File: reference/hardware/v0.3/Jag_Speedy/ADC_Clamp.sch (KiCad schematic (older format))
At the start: 1 part, among them IC10 SP720APP

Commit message: Rationalise level shifting
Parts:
- added IC12: SP720APP, Package_DIP:DIP-16_W7.62mm, symbol Jag_Speedy-rescue:SP720APP-SP720APP-Jag_Speedy-rescue
- added R1, R2, R7, R8: 180k, Resistor_THT:R_Axial_DIN0207_L6.3mm_D2.5mm_P2.54mm_Vertical, symbol Device:R
- added R3, R4, R5, R6: 330k, Resistor_THT:R_Axial_DIN0207_L6.3mm_D2.5mm_P2.54mm_Vertical, symbol Device:R
- added U1: LMV324, Package_DIP:DIP-14_W7.62mm_Socket, symbol Amplifier_Operational:LMV324
- IC10: symbol Jag_Speedy-rescue:SP720APP-SP720APP -> Jag_Speedy-rescue:SP720APP-SP720APP-Jag_Speedy-rescue
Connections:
- net ADCClamp05: now also IC12.1 (IN_1); no longer IC10.5 (IN_5)
- net ADCClamp09: now also IC12.9 (IN_8); no longer IC10.10 (IN_9)
- net ADCClamp10: now also IC12.10 (IN_9); no longer IC10.11 (IN_10)
- net ADCClamp11: now also IC12.11 (IN_10); no longer IC10.12 (IN_11)
- net SignalGnd: now also IC12.8 (V-), R3.2, R4.2, R5.1, R6.1, U1.11 (V-)
- new net: R1.2, R4.1, U1.12 (+)
- new net: R6.2, R8.1, U1.10 (+)
- new net: R2.2, R3.1, U1.5 (+)
- new net: R5.2, R7.1, U1.3 (+)
- new net 3V3: IC12.16 (V+), U1.4 (V+)
- new net Barro-Signal-3.3V: U1.6 (-), U1.7
- new net Barro-Signal-5V: R2.1
- new net MAP-Signal-3.3V: U1.13 (-), U1.14
- new net MAP-Signal-5V: R1.1
- new net O2-Signal-3.3V: U1.1, U1.2 (-)
- new net O2-Signal-5V: R7.2
- new net TPS-Signal-3.3V: U1.8, U1.9 (-)
- new net TPS-Signal-5V: R8.2
- no-connect marks 3 -> 17
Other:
- moved on the sheet: IC10

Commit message: SMD Update
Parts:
- IC10, IC12: footprint Package_DIP:DIP-16_W7.62mm -> Package_SO:SOIC-16_3.9x9.9mm_P1.27mm
- R1, R2, R3, R4, R5, R6, R7, R8: footprint Resistor_THT:R_Axial_DIN0207_L6.3mm_D2.5mm_P2.54mm_Vertical -> Resistor_SMD:R_0805_2012Metric
- U1: footprint Package_DIP:DIP-14_W7.62mm_Socket -> Package_SO:SO-14_5.3x10.2mm_P1.27mm
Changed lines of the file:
@@
 F 0 "IC10" H 2600 1815 50  0000 C CNN
 F 1 "SP720APP" H 2600 1724 50  0000 C CNN
-F 2 "Package_DIP:DIP-16_W7.62mm" H 3050 1650 50  0001 L CNN
+F 2 "Package_SO:SOIC-16_3.9x9.9mm_P1.27mm" H 3050 1650 50  0001 L CNN
 F 3 "https://componentsearchengine.com/Datasheets/1/SP720APP.pdf" H 3050 1550 50  0001 L CNN
 F 4 "TVS Diode Arrays 14 CH DIODE ARRAY" H 3050 1450 50  0001 L CNN "Description"
@@
 F 0 "IC12" H 2600 3115 50  0000 C CNN
 F 1 "SP720APP" H 2600 3024 50  0000 C CNN
-F 2 "Package_DIP:DIP-16_W7.62mm" H 3050 2950 50  0001 L CNN
+F 2 "Package_SO:SOIC-16_3.9x9.9mm_P1.27mm" H 3050 2950 50  0001 L CNN
 F 3 "https://componentsearchengine.com/Datasheets/1/SP720APP.pdf" H 3050 2850 50  0001 L CNN
 F 4 "TVS Diode Arrays 14 CH DIODE ARRAY" H 3050 2750 50  0001 L CNN "Description"
@@
 F 0 "U1" V 6945 3600 50  0000 C CNN
 F 1 "LMV324" V 6854 3600 50  0000 C CNN
-F 2 "Package_DIP:DIP-14_W7.62mm_Socket" H 6800 3700 50  0001 C CNN
+F 2 "Package_SO:SO-14_5.3x10.2mm_P1.27mm" H 6800 3700 50  0001 C CNN
 F 3 "http://www.ti.com/lit/ds/symlink/lmv324.pdf" H 6900 3800 50  0001 C CNN
 	5    6850 3600
@@
 F 0 "U1" V 6354 3180 50  0000 L CNN
 F 1 "LMV324" V 6445 3180 50  0000 L CNN
-F 2 "Package_DIP:DIP-14_W7.62mm_Socket" H 6350 3050 50  0001 C CNN
+F 2 "Package_SO:SO-14_5.3x10.2mm_P1.27mm" H 6350 3050 50  0001 C CNN
 F 3 "http://www.ti.com/lit/ds/symlink/lmv324.pdf" H 6450 3150 50  0001 C CNN
 	4    6400 2950
@@
 F 0 "U1" V 7154 3180 50  0000 L CNN
 F 1 "LMV324" V 7245 3180 50  0000 L CNN
-F 2 "Package_DIP:DIP-14_W7.62mm_Socket" H 7150 3050 50  0001 C CNN
+F 2 "Package_SO:SO-14_5.3x10.2mm_P1.27mm" H 7150 3050 50  0001 C CNN
 F 3 "http://www.ti.com/lit/ds/symlink/lmv324.pdf" H 7250 3150 50  0001 C CNN
 	3    7200 2950
@@
 F 0 "U1" V 6354 2080 50  0000 L CNN
 F 1 "LMV324" V 6445 2080 50  0000 L CNN
-F 2 "Package_DIP:DIP-14_W7.62mm_Socket" H 6350 1950 50  0001 C CNN
+F 2 "Package_SO:SO-14_5.3x10.2mm_P1.27mm" H 6350 1950 50  0001 C CNN
 F 3 "http://www.ti.com/lit/ds/symlink/lmv324.pdf" H 6450 2050 50  0001 C CNN
 	2    6400 1850
@@
 F 0 "U1" V 7154 2080 50  0000 L CNN
 F 1 "LMV324" V 7245 2080 50  0000 L CNN
-F 2 "Package_DIP:DIP-14_W7.62mm_Socket" H 7150 1950 50  0001 C CNN
+F 2 "Package_SO:SO-14_5.3x10.2mm_P1.27mm" H 7150 1950 50  0001 C CNN
 F 3 "http://www.ti.com/lit/ds/symlink/lmv324.pdf" H 7250 2050 50  0001 C CNN
 	1    7200 1850
@@
 F 0 "R8" V 7707 2550 50  0000 C CNN
 F 1 "180k" V 7616 2550 50  0000 C CNN
-F 2 "Resistor_THT:R_Axial_DIN0207_L6.3mm_D2.5mm_P2.54mm_Vertical" V 7430 2550 50  0001 C CNN
+F 2 "Resistor_SMD:R_0805_2012Metric" V 7430 2550 50  0001 C CNN
 F 3 "~" H 7500 2550 50  0001 C CNN
 	1    7500 2550
@@
 F 0 "R6" V 7307 2550 50  0000 C CNN
 F 1 "330k" V 7216 2550 50  0000 C CNN
-F 2 "Resistor_THT:R_Axial_DIN0207_L6.3mm_D2.5mm_P2.54mm_Vertical" V 7030 2550 50  0001 C CNN
+F 2 "Resistor_SMD:R_0805_2012Metric" V 7030 2550 50  0001 C CNN
 F 3 "~" H 7100 2550 50  0001 C CNN
 	1    7100 2550
@@
 F 0 "R4" V 6907 2550 50  0000 C CNN
 F 1 "330k" V 6816 2550 50  0000 C CNN
-F 2 "Resistor_THT:R_Axial_DIN0207_L6.3mm_D2.5mm_P2.54mm_Vertical" V 6630 2550 50  0001 C CNN
+F 2 "Resistor_SMD:R_0805_2012Metric" V 6630 2550 50  0001 C CNN
 F 3 "~" H 6700 2550 50  0001 C CNN
 	1    6700 2550
@@
 F 0 "R1" V 6407 2550 50  0000 C CNN
 F 1 "180k" V 6316 2550 50  0000 C CNN
-F 2 "Resistor_THT:R_Axial_DIN0207_L6.3mm_D2.5mm_P2.54mm_Vertical" V 6130 2550 50  0001 C CNN
+F 2 "Resistor_SMD:R_0805_2012Metric" V 6130 2550 50  0001 C CNN
 F 3 "~" H 6200 2550 50  0001 C CNN
 	1    6200 2550
@@
 F 0 "R3" V 6907 1450 50  0000 C CNN
 F 1 "330k" V 6816 1450 50  0000 C CNN
-F 2 "Resistor_THT:R_Axial_DIN0207_L6.3mm_D2.5mm_P2.54mm_Vertical" V 6630 1450 50  0001 C CNN
+F 2 "Resistor_SMD:R_0805_2012Metric" V 6630 1450 50  0001 C CNN
 F 3 "~" H 6700 1450 50  0001 C CNN
 	1    6700 1450
@@
 F 0 "R2" V 6457 1450 50  0000 C CNN
 F 1 "180k" V 6366 1450 50  0000 C CNN
-F 2 "Resistor_THT:R_Axial_DIN0207_L6.3mm_D2.5mm_P2.54mm_Vertical" V 6180 1450 50  0001 C CNN
+F 2 "Resistor_SMD:R_0805_2012Metric" V 6180 1450 50  0001 C CNN
 F 3 "~" H 6250 1450 50  0001 C CNN
 	1    6250 1450
@@
 F 0 "R7" V 7707 1450 50  0000 C CNN
 F 1 "180k" V 7616 1450 50  0000 C CNN
-F 2 "Resistor_THT:R_Axial_DIN0207_L6.3mm_D2.5mm_P2.54mm_Vertical" V 7430 1450 50  0001 C CNN
+F 2 "Resistor_SMD:R_0805_2012Metric" V 7430 1450 50  0001 C CNN
 F 3 "~" H 7500 1450 50  0001 C CNN
 	1    7500 1450
@@
 F 0 "R5" V 7307 1450 50  0000 C CNN
 F 1 "330k" V 7216 1450 50  0000 C CNN
-F 2 "Resistor_THT:R_Axial_DIN0207_L6.3mm_D2.5mm_P2.54mm_Vertical" V 7030 1450 50  0001 C CNN
+F 2 "Resistor_SMD:R_0805_2012Metric" V 7030 1450 50  0001 C CNN
 F 3 "~" H 7100 1450 50  0001 C CNN
 	1    7100 1450

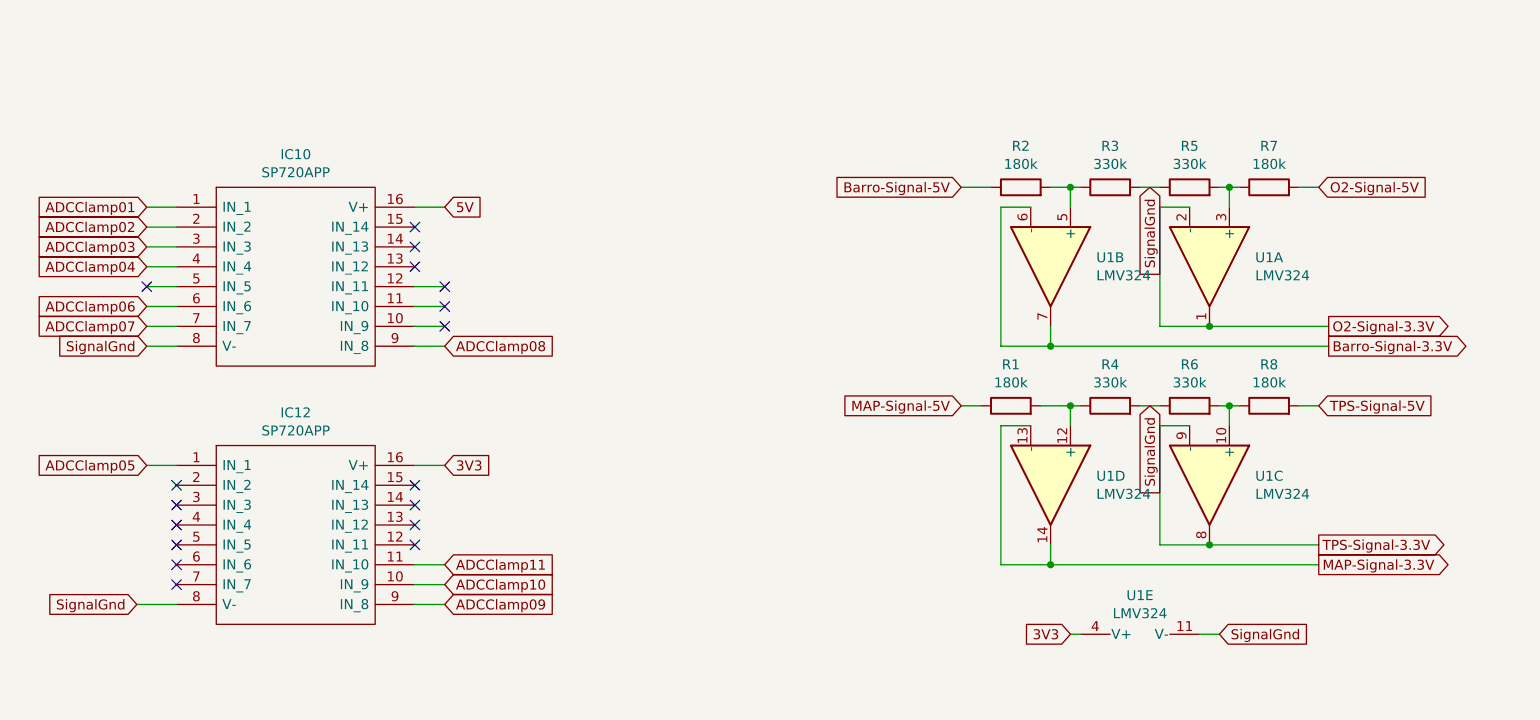
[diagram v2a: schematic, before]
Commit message: VR Conditioner
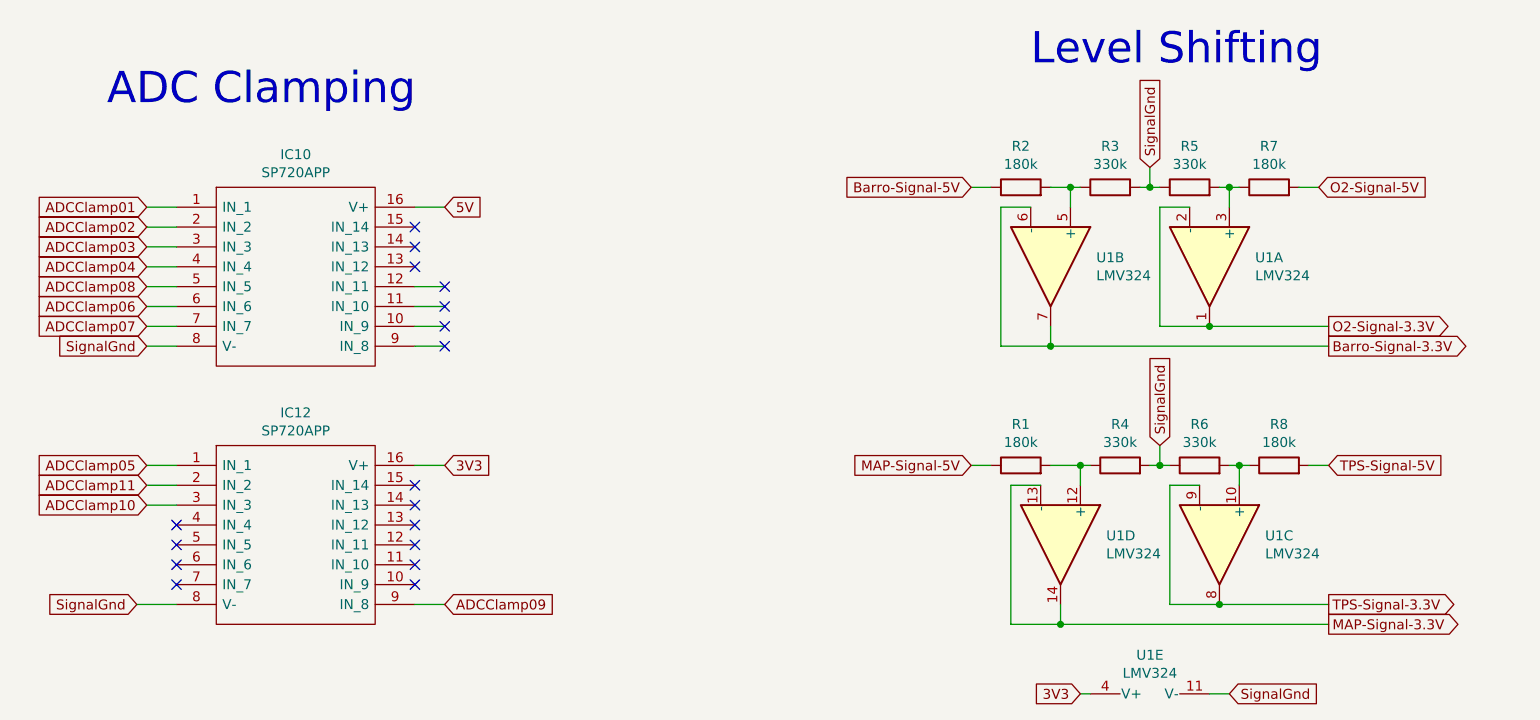
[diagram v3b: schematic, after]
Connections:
- net ADCClamp08: now also IC10.5 (IN_5); no longer IC10.9 (IN_8)
- net ADCClamp10: now also IC12.3 (IN_3); no longer IC12.10 (IN_9)
- net ADCClamp11: now also IC12.2 (IN_2); no longer IC12.11 (IN_10)
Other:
- note added: "ADC Clamping"
- note added: "Level Shifting"
- moved on the sheet: R1, R4, R6, R8, U1C, U1D, U1E
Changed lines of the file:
@@
 Text GLabel 1850 2150 0    50   Input ~ 0
 ADCClamp07
-Text GLabel 3350 2250 2    50   Input ~ 0
+Text GLabel 1850 1950 0    50   Input ~ 0
 ADCClamp08
 Text GLabel 3350 3550 2    50   Input ~ 0
 ADCClamp09
-Text GLabel 3350 3450 2    50   Input ~ 0
+Text GLabel 1850 3050 0    50   Input ~ 0
 ADCClamp10
-Text GLabel 3350 3350 2    50   Input ~ 0
+Text GLabel 1850 2950 0    50   Input ~ 0
 ADCClamp11
 $Comp
@@
 Text GLabel 3350 2850 2    50   Input ~ 0
 3V3
-NoConn ~ 1850 1950
 Wire Wire Line
 	3350 2850 3200 2850
@@
 NoConn ~ 3350 2150
 NoConn ~ 3350 2050
-Wire Wire Line
-	3350 3450 3200 3450
-Wire Wire Line
-	3350 3350 3200 3350
 NoConn ~ 3350 1950
 $Comp
 L Amplifier_Operational:LMV324 U?
 U 5 1 5F0A9466
-P 6850 3600
+P 6900 3900
 AR Path="/5F0A9466" Ref="U?"  Part="5"
 AR Path="/5EF0F56B/5F0A9466" Ref="U1"  Part="5"
-F 0 "U1" V 6945 3600 50  0000 C CNN
-F 1 "LMV324" V 6854 3600 50  0000 C CNN
-F 2 "Package_SO:SO-14_5.3x10.2mm_P1.27mm" H 6800 3700 50  0001 C CNN
-F 3 "http://www.ti.com/lit/ds/symlink/lmv324.pdf" H 6900 3800 50  0001 C CNN
-	5    6850 3600
+F 0 "U1" V 6995 3900 50  0000 C CNN
+F 1 "LMV324" V 6904 3900 50  0000 C CNN
+F 2 "Package_SO:SO-14_5.3x10.2mm_P1.27mm" H 6850 4000 50  0001 C CNN
+F 3 "http://www.ti.com/lit/ds/symlink/lmv324.pdf" H 6950 4100 50  0001 C CNN
+	5    6900 3900
 	0    -1   -1   0
 $EndComp
@@
 L Amplifier_Operational:LMV324 U?
 U 4 1 5F0A946C
-P 6400 2950
+P 6450 3250
 AR Path="/5F0A946C" Ref="U?"  Part="4"
 AR Path="/5EF0F56B/5F0A946C" Ref="U1"  Part="4"
-F 0 "U1" V 6354 3180 50  0000 L CNN
-F 1 "LMV324" V 6445 3180 50  0000 L CNN
-F 2 "Package_SO:SO-14_5.3x10.2mm_P1.27mm" H 6350 3050 50  0001 C CNN
-F 3 "http://www.ti.com/lit/ds/symlink/lmv324.pdf" H 6450 3150 50  0001 C CNN
-	4    6400 2950
+F 0 "U1" V 6404 3480 50  0000 L CNN
+F 1 "LMV324" V 6495 3480 50  0000 L CNN
+F 2 "Package_SO:SO-14_5.3x10.2mm_P1.27mm" H 6400 3350 50  0001 C CNN
+F 3 "http://www.ti.com/lit/ds/symlink/lmv324.pdf" H 6500 3450 50  0001 C CNN
+	4    6450 3250
 	0    1    1    0
 $EndComp
@@
 L Amplifier_Operational:LMV324 U?
 U 3 1 5F0A9472
-P 7200 2950
+P 7250 3250
 AR Path="/5F0A9472" Ref="U?"  Part="3"
 AR Path="/5EF0F56B/5F0A9472" Ref="U1"  Part="3"
-F 0 "U1" V 7154 3180 50  0000 L CNN
-F 1 "LMV324" V 7245 3180 50  0000 L CNN
-F 2 "Package_SO:SO-14_5.3x10.2mm_P1.27mm" H 7150 3050 50  0001 C CNN
-F 3 "http://www.ti.com/lit/ds/symlink/lmv324.pdf" H 7250 3150 50  0001 C CNN
-	3    7200 2950
+F 0 "U1" V 7204 3480 50  0000 L CNN
+F 1 "LMV324" V 7295 3480 50  0000 L CNN
+F 2 "Package_SO:SO-14_5.3x10.2mm_P1.27mm" H 7200 3350 50  0001 C CNN
+F 3 "http://www.ti.com/lit/ds/symlink/lmv324.pdf" H 7300 3450 50  0001 C CNN
+	3    7250 3250
 	0    1    1    0
 $EndComp
@@
 Text GLabel 7750 1450 2    50   Input ~ 0
 O2-Signal-5V
-Text GLabel 7750 3250 2    50   Output ~ 0
+Text GLabel 7800 3550 2    50   Output ~ 0
 TPS-Signal-3.3V
 $Comp
 L Device:R R?
 U 1 1 5F0A9487
-P 7500 2550
+P 7550 2850
 AR Path="/5F0A9487" Ref="R?"  Part="1"
 AR Path="/5EF0F56B/5F0A9487" Ref="R8"  Part="1"
-F 0 "R8" V 7707 2550 50  0000 C CNN
-F 1 "180k" V 7616 2550 50  0000 C CNN
-F 2 "Resistor_SMD:R_0805_2012Metric" V 7430 2550 50  0001 C CNN
-F 3 "~" H 7500 2550 50  0001 C CNN
-	1    7500 2550
+F 0 "R8" V 7757 2850 50  0000 C CNN
+F 1 "180k" V 7666 2850 50  0000 C CNN
+F 2 "Resistor_SMD:R_0805_2012Metric" V 7480 2850 50  0001 C CNN
+F 3 "~" H 7550 2850 50  0001 C CNN
+	1    7550 2850
 	0    -1   -1   0
 $EndComp
@@
 L Device:R R?
 U 1 1 5F0A948D
-P 7100 2550
+P 7150 2850
 AR Path="/5F0A948D" Ref="R?"  Part="1"
 AR Path="/5EF0F56B/5F0A948D" Ref="R6"  Part="1"
-F 0 "R6" V 7307 2550 50  0000 C CNN
-F 1 "330k" V 7216 2550 50  0000 C CNN
-F 2 "Resistor_SMD:R_0805_2012Metric" V 7030 2550 50  0001 C CNN
-F 3 "~" H 7100 2550 50  0001 C CNN
-	1    7100 2550
+F 0 "R6" V 7357 2850 50  0000 C CNN
+F 1 "330k" V 7266 2850 50  0000 C CNN
+F 2 "Resistor_SMD:R_0805_2012Metric" V 7080 2850 50  0001 C CNN
+F 3 "~" H 7150 2850 50  0001 C CNN
+	1    7150 2850
 	0    -1   -1   0
 $EndComp
@@
 L Device:R R?
 U 1 1 5F0A9493
-P 6700 2550
+P 6750 2850
 AR Path="/5F0A9493" Ref="R?"  Part="1"
 AR Path="/5EF0F56B/5F0A9493" Ref="R4"  Part="1"
-F 0 "R4" V 6907 2550 50  0000 C CNN
-F 1 "330k" V 6816 2550 50  0000 C CNN
-F 2 "Resistor_SMD:R_0805_2012Metric" V 6630 2550 50  0001 C CNN
-F 3 "~" H 6700 2550 50  0001 C CNN
-	1    6700 2550
+F 0 "R4" V 6957 2850 50  0000 C CNN
+F 1 "330k" V 6866 2850 50  0000 C CNN
+F 2 "Resistor_SMD:R_0805_2012Metric" V 6680 2850 50  0001 C CNN
+F 3 "~" H 6750 2850 50  0001 C CNN
+	1    6750 2850
 	0    -1   -1   0
 $EndComp
@@
 L Device:R R?
 U 1 1 5F0A9499
-P 6200 2550
+P 6250 2850
 AR Path="/5F0A9499" Ref="R?"  Part="1"
 AR Path="/5EF0F56B/5F0A9499" Ref="R1"  Part="1"
-F 0 "R1" V 6407 2550 50  0000 C CNN
-F 1 "180k" V 6316 2550 50  0000 C CNN
-F 2 "Resistor_SMD:R_0805_2012Metric" V 6130 2550 50  0001 C CNN
-F 3 "~" H 6200 2550 50  0001 C CNN
-	1    6200 2550
-	0    -1   -1   0
-$EndComp
-Text GLabel 5950 2550 0    50   Input ~ 0
+F 0 "R1" V 6457 2850 50  0000 C CNN
+F 1 "180k" V 6366 2850 50  0000 C CNN
+F 2 "Resistor_SMD:R_0805_2012Metric" V 6180 2850 50  0001 C CNN
+F 3 "~" H 6250 2850 50  0001 C CNN
+	1    6250 2850
+	0    -1   -1   0
+$EndComp
+Text GLabel 6000 2850 0    50   Input ~ 0
 MAP-Signal-5V
 Wire Wire Line
-	5950 2550 6050 2550
-Wire Wire Line
-	6350 2550 6500 2550
-Wire Wire Line
-	7250 2550 7300 2550
-Wire Wire Line
-	7300 2650 7300 2550
-Connection ~ 7300 2550
-Wire Wire Line
-	7300 2550 7350 2550
-Wire Wire Line
-	6500 2650 6500 2550
-Connection ~ 6500 2550
-Wire Wire Line
-	6500 2550 6550 2550
-Text GLabel 6500 3700 0    50   Input ~ 0
+	6000 2850 6100 2850
+Wire Wire Line
+	6400 2850 6550 2850
+Wire Wire Line
+	7300 2850 7350 2850
+Wire Wire Line
+	7350 2950 7350 2850
+Connection ~ 7350 2850
+Wire Wire Line
+	7350 2850 7400 2850
+Wire Wire Line
+	6550 2950 6550 2850
+Connection ~ 6550 2850
+Wire Wire Line
+	6550 2850 6600 2850
+Text GLabel 6550 4000 0    50   Input ~ 0
 3V3
 Wire Wire Line
-	6500 3700 6550 3700
-Wire Wire Line
-	6400 3350 6400 3250
-Wire Wire Line
-	7100 2650 6950 2650
-Wire Wire Line
-	6950 2650 6950 3250
-Wire Wire Line
-	6950 3250 7200 3250
-Wire Wire Line
-	6300 2650 6150 2650
-Wire Wire Line
-	6150 2650 6150 3350
-Wire Wire Line
-	6150 3350 6400 3350
-Connection ~ 6400 3350
-Wire Wire Line
-	7750 3250 7200 3250
-Connection ~ 7200 3250
-Wire Wire Line
-	6400 3350 7750 3350
-Text GLabel 5950 1450 0    50   Input ~ 0
+	6550 4000 6600 4000
+Wire Wire Line
+	6450 3650 6450 3550
+Wire Wire Line
+	7150 2950 7000 2950
+Wire Wire Line
+	7000 2950 7000 3550
+Wire Wire Line
+	7000 3550 7250 3550
+Wire Wire Line
+	6350 2950 6200 2950
+Wire Wire Line
+	6200 2950 6200 3650
+Wire Wire Line
+	6200 3650 6450 3650
+Connection ~ 6450 3650
+Wire Wire Line
+	7800 3550 7250 3550
+Connection ~ 7250 3550
+Wire Wire Line
+	6450 3650 7800 3650
+Text GLabel 6000 1450 0    50   Input ~ 0
 Barro-Signal-5V
 Wire Wire Line
-	7650 2550 7750 2550
-Text GLabel 7750 2550 2    50   Input ~ 0
+	7700 2850 7800 2850
+Text GLabel 7800 2850 2    50   Input ~ 0
 TPS-Signal-5V
 Text GLabel 7800 2250 2    50   Output ~ 0
@@
 $EndComp
 Wire Wire Line
-	5950 1450 6100 1450
-Wire Wire Line
 	6400 1450 6500 1450
 Wire Wire Line
@@
 Wire Wire Line
 	7750 1450 7650 1450
-Text GLabel 7250 3700 2    50   Input ~ 0
+Text GLabel 7300 4000 2    50   Input ~ 0
 SignalGnd
 Wire Wire Line
-	7250 3700 7150 3700
-Wire Wire Line
-	6850 2550 6950 2550
-Text GLabel 6900 2550 3    50   Input ~ 0
+	7300 4000 7200 4000
+Wire Wire Line
+	6900 2850 6950 2850
+Text GLabel 6950 2750 1    50   Input ~ 0
 SignalGnd
-Text GLabel 6900 1450 3    50   Input ~ 0
+Text GLabel 6900 1350 1    50   Input ~ 0
 SignalGnd
-Text GLabel 7750 3350 2    50   Output ~ 0
+Text GLabel 7800 3650 2    50   Output ~ 0
 MAP-Signal-3.3V
 Wire Wire Line
@@
 	6400 2250 7800 2250
 Wire Wire Line
-	6850 1450 6950 1450
-NoConn ~ 2000 2950
-NoConn ~ 2000 3050
+	6850 1450 6900 1450
 NoConn ~ 2000 3150
 NoConn ~ 2000 3250
@@
 Wire Wire Line
 	1800 3550 2000 3550
+Wire Wire Line
+	2000 2950 1850 2950
+Wire Wire Line
+	1850 3050 2000 3050
+NoConn ~ 3200 3450
+NoConn ~ 3200 3350
+NoConn ~ 3350 2250
+Wire Wire Line
+	6900 1350 6900 1450
+Connection ~ 6900 1450
+Wire Wire Line
+	6900 1450 6950 1450
+Wire Wire Line
+	6950 2750 6950 2850
+Connection ~ 6950 2850
+Wire Wire Line
+	6950 2850 7000 2850
+Wire Wire Line
+	6000 1450 6100 1450
+Text Notes 1650 1050 0    157  ~ 0
+ADC Clamping
+Text Notes 6300 850  0    157  ~ 0
+Level Shifting
 $EndSCHEMATC
